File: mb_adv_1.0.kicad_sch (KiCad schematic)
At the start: 5 parts, among them SW2 SW_SP3T, U2 gba_link_cable, U3 BOB-12009

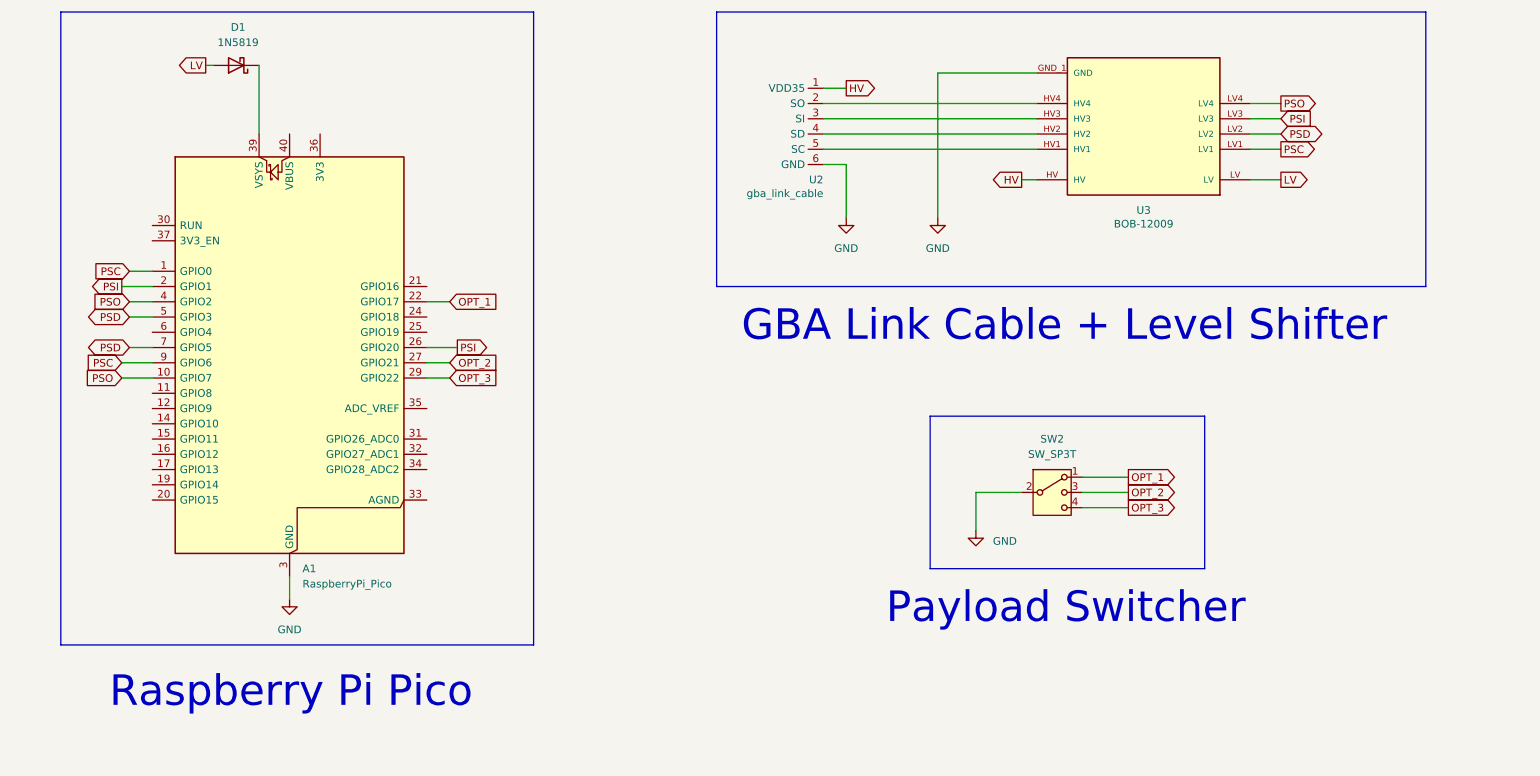
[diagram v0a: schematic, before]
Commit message: add microSD card
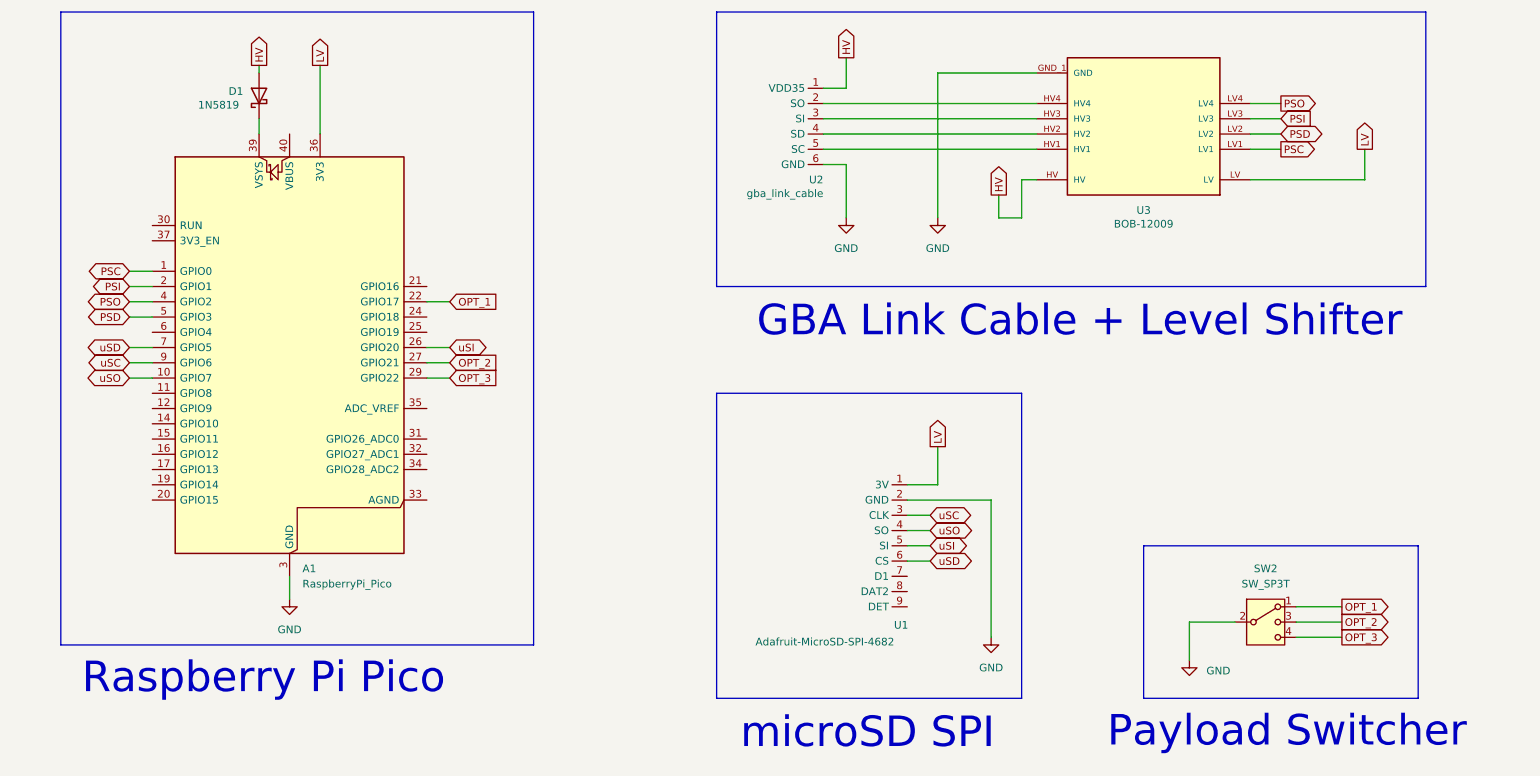
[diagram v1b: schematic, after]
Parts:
- added U1: Adafruit-MicroSD-SPI-4682, adafruit:adafruit_4682, symbol adafruit_4682:microSD_SPI_SDIO_4682
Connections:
- net GND: now also U1.2 (GND)
- net HV: now also D1.2 (A)
- net LV: now also A1.36 (3V3), U1.1 (3V); no longer D1.2 (A)
- net PSC: no longer A1.9 (GPIO6)
- net PSD: no longer A1.7 (GPIO5)
- net PSI: no longer A1.26 (GPIO20)
- net PSO: no longer A1.10 (GPIO7)
- new net uSC: A1.9 (GPIO6), U1.3 (CLK)
- new net uSD: A1.7 (GPIO5), U1.6 (CS)
- new net uSI: A1.26 (GPIO20), U1.5 (SI)
- new net uSO: A1.10 (GPIO7), U1.4 (SO)
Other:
- note added: "microSD SPI"
- moved on the sheet: D1, SW2
